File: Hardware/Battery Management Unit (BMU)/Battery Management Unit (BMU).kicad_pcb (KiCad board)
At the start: 4 copper layers, 105 x 66 mm, 90 parts, among them IC1 STM32C092RCT6, J1 HIGH SIDE, J10 SHUNT, J11 Conn_ST_STDC14, J2 LOW SIDE, J3 POWER, J4 GPIO, J5 pin header, J6 CAN, J7 5V, J8 3V3, J9 GND, Q1 DMP3099L, SW1 Power Switch, SW2 SW_Push, T1 CEP99-102, T2 CEP99-102, U1 OKI-78SR-5_1.5-W36-C, U2 TLV75533PDBV, U3 PESD5V0L2BT, U4 PESD5V0L2BT, U5 BQ79600PWRQ1, U6 MCP2562FDT-H_SN

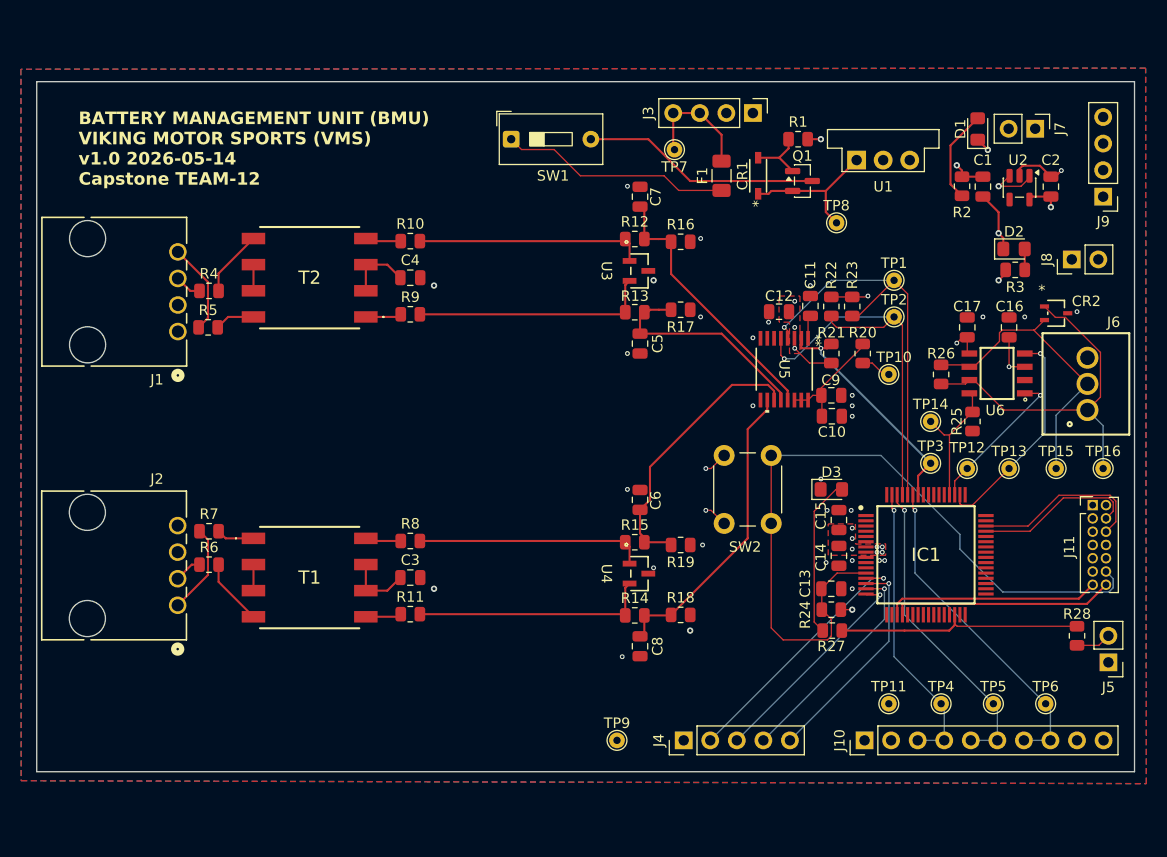
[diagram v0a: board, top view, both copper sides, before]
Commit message: finish! update bmu layout+BOM
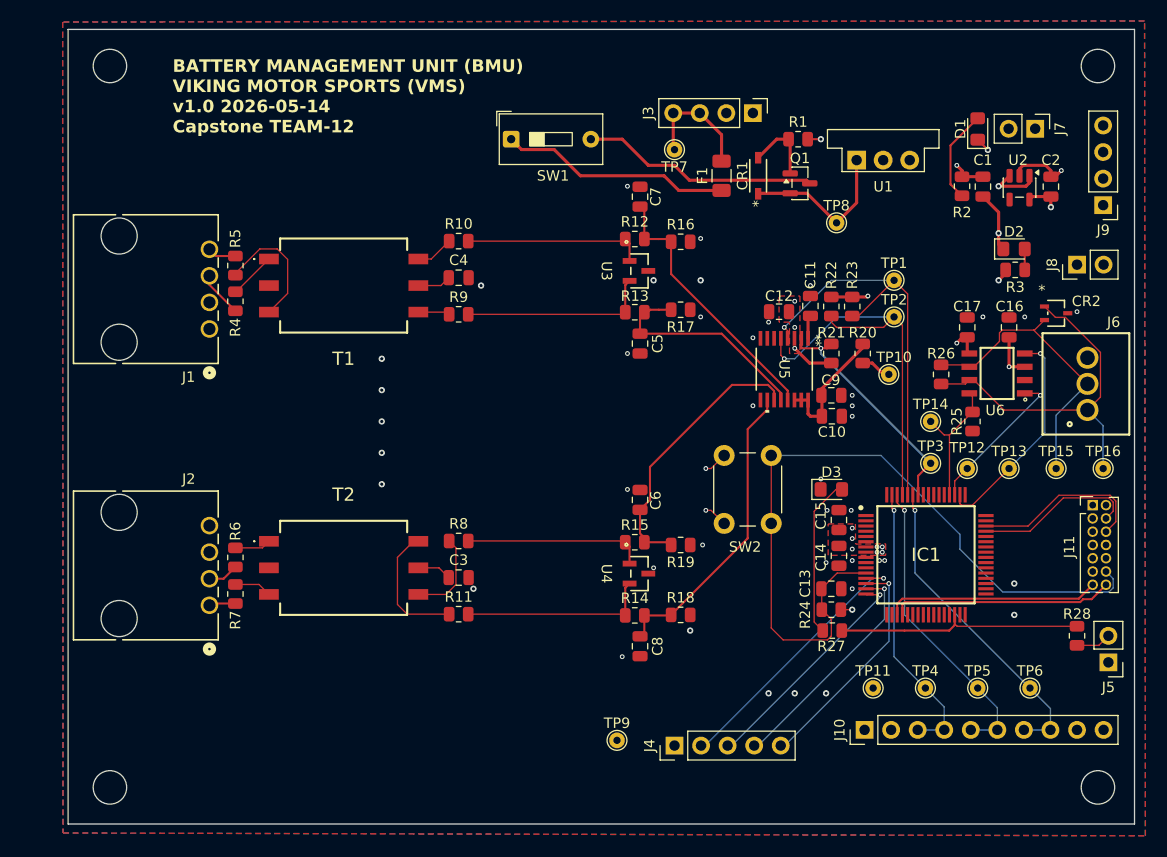
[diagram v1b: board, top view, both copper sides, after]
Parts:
- added REF**: MountingHole_3.2mm_M3, MountingHole:MountingHole_3.2mm_M3, F.Cu at (185.0, 138.5)
- added REF**: MountingHole_3.2mm_M3, MountingHole:MountingHole_3.2mm_M3, F.Cu at (90.5, 138.5)
- added REF**: MountingHole_3.2mm_M3, MountingHole:MountingHole_3.2mm_M3, F.Cu at (185.0, 69.5)
- added REF**: MountingHole_3.2mm_M3, MountingHole:MountingHole_3.2mm_M3, F.Cu at (90.5, 69.5)
- C12, C9: value 0.1u -> 100n
- Q1: value DMP3099L -> AO3401A
- T1, T2: value CEP99-102 -> HM2147NLT; footprint Footprints:CEP99102 -> Footprints:HM2147NLT
- moved T1 28.1 mm to (112.9, 90.5), turned to -90 degrees
- moved T2 27.9 mm to (112.9, 117.5), turned to -90 degrees
- moved R7 6.51 mm to (102.5, 120.0), turned to 90 degrees
- moved R5 6.46 mm to (102.5, 88.6), turned to -90 degrees
- moved C3 4.62 mm to (123.9, 118.4)
- moved C4 4.62 mm to (123.9, 89.8)
- moved R10 4.62 mm to (123.9, 86.2)
- moved R11 4.62 mm to (123.9, 121.9)
- moved R8 4.62 mm to (123.9, 114.9)
- moved R9 4.62 mm to (123.9, 93.2)
- moved J2 3.04 mm to (100.0, 121.1)
- moved J1 3.03 mm to (100.0, 94.6)
- moved R4 2.71 mm to (102.5, 92.0), turned to 90 degrees
- moved R6 2.61 mm to (102.5, 116.5), turned to 90 degrees
- moved TP11 2.12 mm to (163.5, 129.0)
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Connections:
- C3 pad 1: Net-(C3-Pad1) -> Net-(T2-SEC_2)
- C4 pad 1: Net-(C4-Pad1) -> Net-(T1-SEC_2)
- R10 pad 1: Net-(R10-Pad1) -> Net-(T1-SEC_3)
- R11 pad 1: Net-(R11-Pad1) -> Net-(T2-SEC_3)
- R4 pad 2: Net-(R4-Pad2) -> Net-(T1-PRI_1)
- R5 pad 2: Net-(R5-Pad2) -> Net-(T1-PRI_3)
- R6 pad 2: Net-(R6-Pad2) -> Net-(T2-PRI_1)
- R7 pad 2: Net-(R7-Pad2) -> Net-(T2-PRI_3)
- R8 pad 1: Net-(R8-Pad1) -> Net-(T2-SEC_1)
- R9 pad 1: Net-(R9-Pad1) -> Net-(T1-SEC_1)
- T1 pad 1: Net-(R7-Pad2) -> Net-(T1-PRI_1)
- T1 pad 2: Net-(T1-Pad2) -> unconnected-(T1-PRI_2-Pad2)
- T1 pad 3: Net-(T1-Pad2) -> Net-(T1-PRI_3)
- T1 pad 4: Net-(R6-Pad2) -> Net-(T1-SEC_1)
- T1 pad 5: Net-(R11-Pad1) -> Net-(T1-SEC_2)
- T1 pad 6: Net-(C3-Pad1) -> Net-(T1-SEC_3)
- T2 pad 1: Net-(R9-Pad1) -> Net-(T2-PRI_1)
- T2 pad 2: Net-(C4-Pad1) -> unconnected-(T2-PRI_2-Pad2)
- T2 pad 3: Net-(C4-Pad1) -> Net-(T2-PRI_3)
- T2 pad 4: Net-(R10-Pad1) -> Net-(T2-SEC_1)
- T2 pad 5: Net-(R4-Pad2) -> Net-(T2-SEC_2)
- T2 pad 6: Net-(T2-Pad6) -> Net-(T2-SEC_3)
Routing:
- net Net-(T2-SEC_3): track 0.00 -> 12.5 mm
- net Net-(T1-PRI_3): track 0.00 -> 12.3 mm
- net Net-(T2-SEC_1): track 0.00 -> 8.42 mm
- net Net-(R4-Pad2): track 6.39 -> 0.00 mm
- net Net-(R6-Pad2): track 6.37 -> 0.00 mm
- net Net-(C4-Pad1): track 6.32 -> 0.00 mm
- net Net-(C3-Pad1): track 6.32 -> 0.00 mm
- net /LOW COMLN: track 8.62 -> 2.55 mm
- net /High COMHN: track 8.79 -> 2.75 mm
- net /BMU-COM Bridge/COMLP_OPT: track 22.9 -> 18.3 mm
- net /BMU-COM Bridge/COMLN_OPT: track 21.9 -> 17.3 mm
- net /BMU-COM Bridge/COMHP_OPT: track 22.0 -> 17.4 mm
- net /BMU-COM Bridge/COMHN_OPT: track 22.9 -> 18.3 mm
- net Net-(T1-PRI_1): track 0.00 -> 4.51 mm
- net /BMU-POWER/VIN_PROTECTED: track 14.2 -> 18.5 mm
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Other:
- board size 105 x 66 mm -> 102 x 76 mm
